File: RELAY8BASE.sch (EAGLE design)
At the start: 75 parts, among them IC1 MCP23017SO, J1 Analog, J2 POWER, J3 Digital_0_7, J4 M100.1, J5 ICSPPTH, J7 PWR SELECT, Q1 2N7002, Q2 2N7002, Q3 2N7002, Q4 2N7002, Q5 2N7002, Q6 2N7002, Q7 2N7002, Q8 2N7002

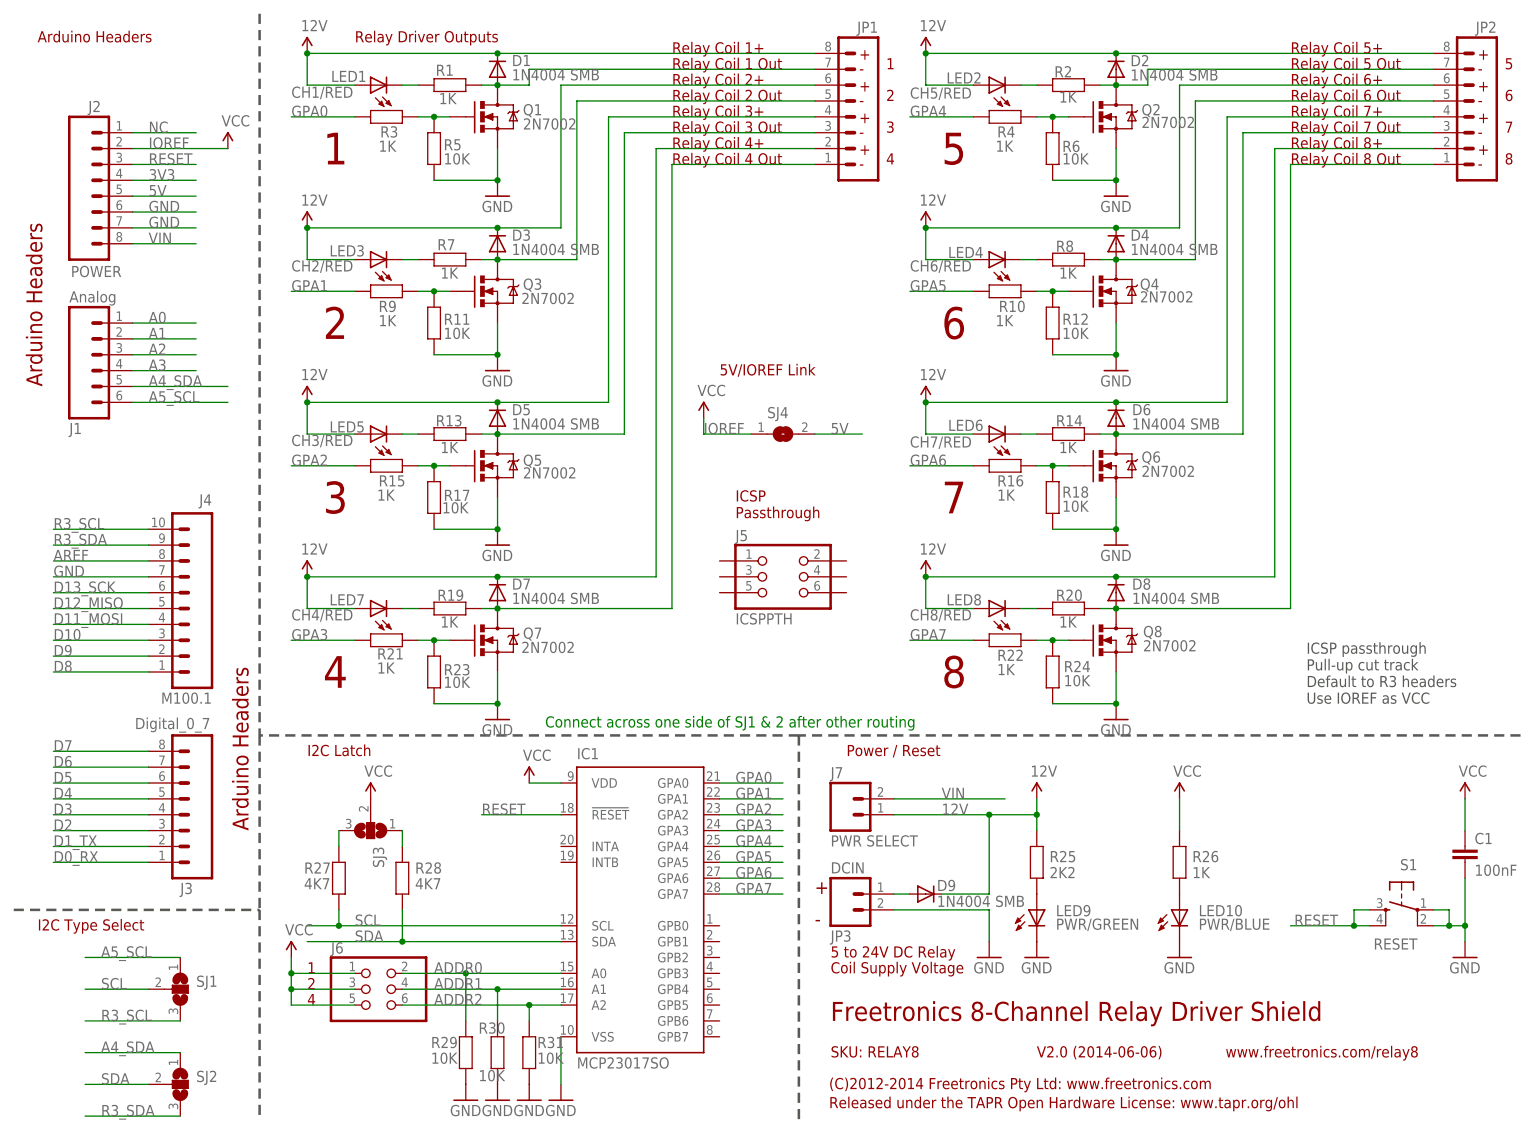
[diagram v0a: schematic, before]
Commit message: Layout for v1.0 release
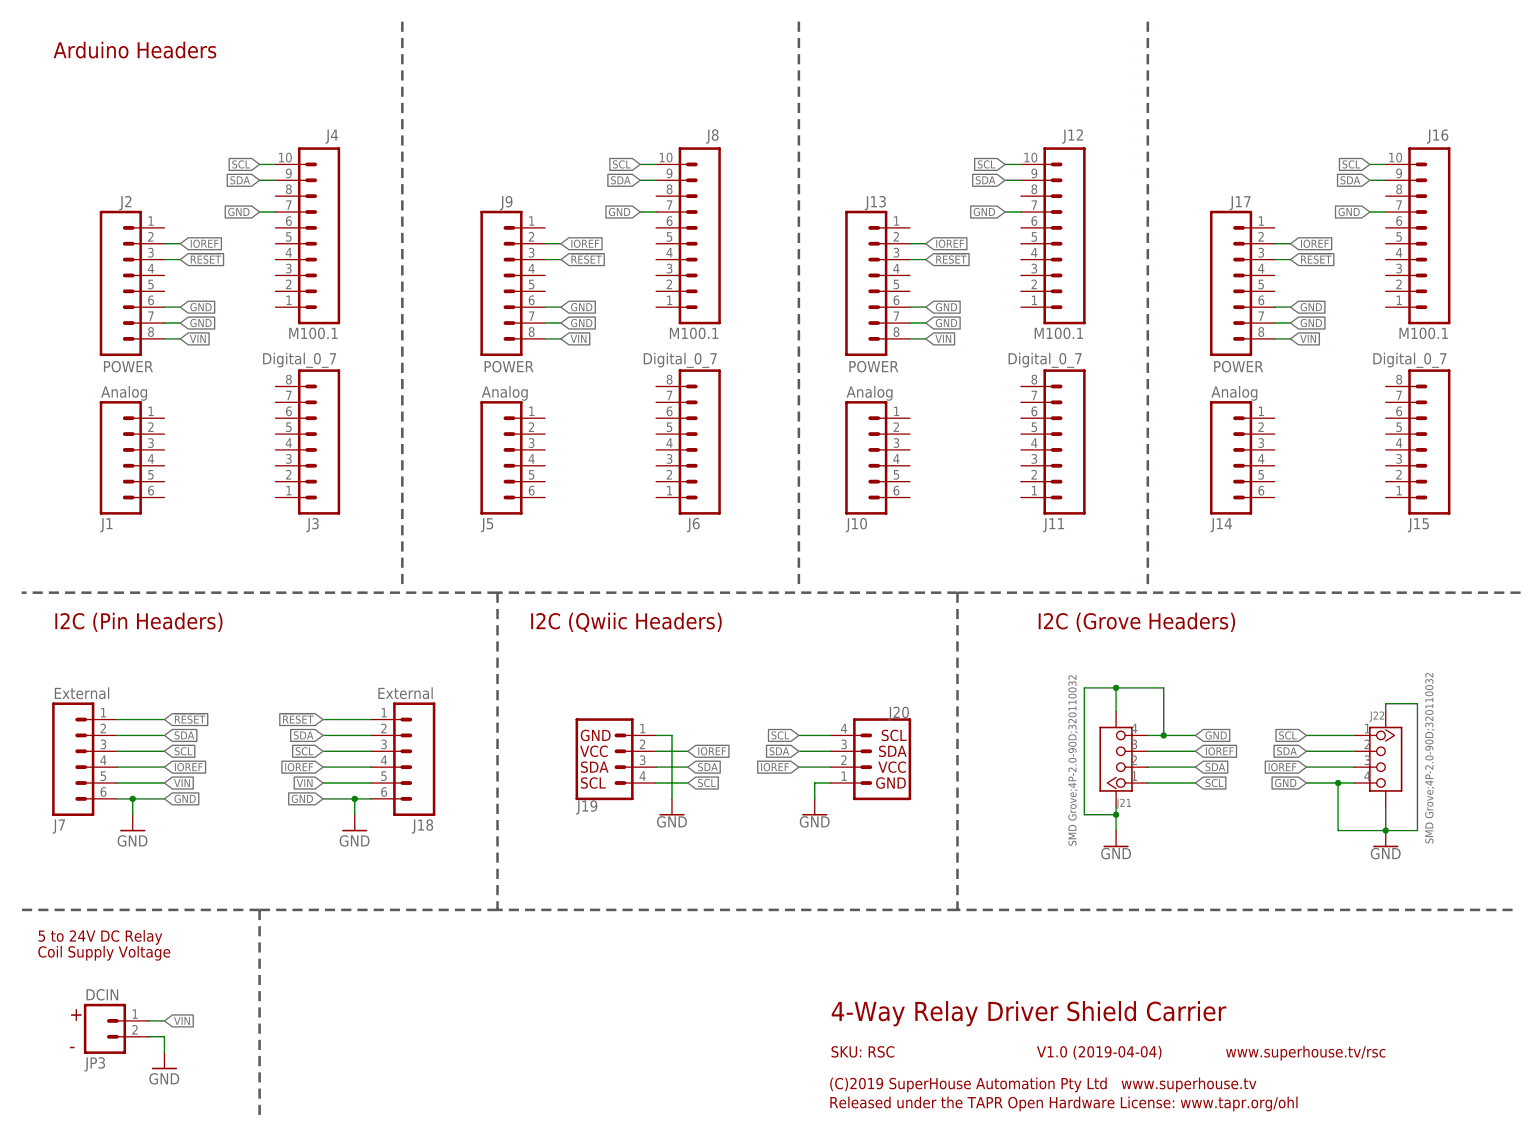
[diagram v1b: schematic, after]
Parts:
- removed C1: 100nF, freetronics-original:CAP0603
- removed D1, D2, D3, D4, D5, D6, D7, D8, D9: 1N4004 SMB, freetronics-master-v1.1:DIODESMB
- removed IC1: MCP23017SO, microchip:MCP23017SO
- removed JP1, JP2: (no value), freetronics-master-v1:M08
- removed LED1: CH1/RED, freetronics-master-v1:LED0603
- removed LED10: PWR/BLUE, freetronics-master-v1:LED0603
- removed LED2: CH5/RED, freetronics-master-v1:LED0603
- removed LED3: CH2/RED, freetronics-master-v1:LED0603
- removed LED4: CH6/RED, freetronics-master-v1:LED0603
- removed LED5: CH3/RED, freetronics-master-v1:LED0603
- removed LED6: CH7/RED, freetronics-master-v1:LED0603
- removed LED7: CH4/RED, freetronics-master-v1:LED0603
- removed LED8: CH8/RED, freetronics-master-v1:LED0603
- removed LED9: PWR/GREEN, freetronics-master-v1:LED0603
- removed Q1, Q2, Q3, Q4, Q5, Q6, Q7, Q8: 2N7002, freetronics-master-v1:MOSFET-NCHANNELSMD
- removed R1, R10, R13, R14, R15, R16, R19, R2, R20, R21, R22, R26, R3, R4, R7, R8, R9: 1K, freetronics-master-v1:RESISTOR0603
- removed R11, R12, R17, R18, R23, R24, R29, R30, R31, R5, R6: 10K, freetronics-master-v1:RESISTOR0603
- removed R25: 2K2, freetronics-master-v1:RESISTOR0603
- removed R27, R28: 4K7, freetronics-master-v1:RESISTOR0603
- removed S1: RESET, freetronics-original:TAC_SWITCHSMD
- removed SJ1, SJ2, SJ3: (no value), freetronics-master-v1.1:SJ2W
- removed SJ4: (no value), freetronics-jon:SJN
- added J10, J14: Analog, freetronics:M06SIP
- added J11, J15: Digital_0_7, freetronics:M08
- added J12, J16, J8: M100.1, freetronics-original:M100.1
- added J13, J17, J9: POWER, freetronics:M08
- added J18: External, freetronics:M06SIP
- added J19, J20: (no value), SparkFun-Connectors:QWIIC_CONNECTORJS-1MM
- added J21, J22: SMD Grove;4P-2.0-90D;320110032, Connector-new:GROVE-CONNECTOR-SMD'90D'
- J5: value ICSPPTH -> Analog; device freetronics-jon:ICSPPTH -> freetronics:M06SIP
- J6: value (none) -> Digital_0_7; device freetronics-master-v1.1:PINHD-2X3 -> freetronics:M08
- J7: value PWR SELECT -> External; device SparkFun:M02PTH -> freetronics:M06SIP
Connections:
- removed net 12V: D1.C, D2.C, D3.C, D4.C, D5.C, D6.C, D7.C, D8.C, D9.C, J7.1, JP1.2, JP1.4, JP1.6, JP1.8, JP2.2, JP2.4, JP2.6, JP2.8, LED1.A, LED2.A, LED3.A, LED4.A, LED5.A, LED6.A, LED7.A, LED8.A, R25.2
- removed net 3V3: J2.4
- removed net 5V: J2.5, SJ4.2
- removed net A0: J1.1
- removed net A1: J1.2
- removed net A2: J1.3
- removed net A3: J1.4
- removed net A4_SDA: J1.5, SJ2.1
- removed net A5_SCL: J1.6, SJ1.1
- removed net ADDR0: IC1.A0, J6.2, R29.2
- removed net ADDR1: IC1.A1, J6.4, R30.2
- removed net ADDR2: IC1.A2, J6.6, R31.2
- removed net AREF: J4.8
- removed net D0_RX: J3.1
- removed net D10: J4.3
- removed net D11_MOSI: J4.4
- removed net D12_MISO: J4.5
- removed net D13_SCK: J4.6
- removed net D1_TX: J3.2
- removed net D2: J3.3
- removed net D3: J3.4
- removed net D4: J3.5
- removed net D5: J3.6
- removed net D6: J3.7
- removed net D7: J3.8
- removed net D8: J4.1
- removed net D9: J4.2
- removed net GPA0: IC1.GPA0, R3.2
- removed net GPA1: IC1.GPA1, R9.2
- removed net GPA2: IC1.GPA2, R15.2
- removed net GPA3: IC1.GPA3, R21.2
- removed net GPA4: IC1.GPA4, R4.2
- removed net GPA5: IC1.GPA5, R10.2
- removed net GPA6: IC1.GPA6, R16.2
- removed net GPA7: IC1.GPA7, R22.2
- removed net N$1: Q1.G, R3.1, R5.2
- removed net N$10: Q5.G, R15.1, R17.2
- removed net N$11: D7.A, JP1.1, Q7.D, R19.2
- removed net N$12: Q7.G, R21.1, R23.2
- removed net N$13: D2.A, JP2.7, Q2.D, R2.2
- removed net N$14: Q2.G, R4.1, R6.2
- removed net N$15: D4.A, JP2.5, Q4.D, R8.2
- removed net N$16: Q4.G, R10.1, R12.2
- removed net N$17: D6.A, JP2.3, Q6.D, R14.2
- removed net N$18: Q6.G, R16.1, R18.2
- removed net N$19: D8.A, JP2.1, Q8.D, R20.2
- removed net N$20: Q8.G, R22.1, R24.2
- removed net N$21: LED3.C, R7.1
- removed net N$22: LED7.C, R19.1
- removed net N$23: LED5.C, R13.1
- removed net N$24: LED1.C, R1.1
- removed net N$25: LED2.C, R2.1
- removed net N$26: LED4.C, R8.1
- removed net N$27: LED6.C, R14.1
- removed net N$28: LED8.C, R20.1
- removed net N$3: D3.A, JP1.5, Q3.D, R7.2
- removed net N$4: LED9.A, R25.1
- removed net N$41: D9.A, JP3.1
- removed net N$42: R27.2, SJ3.3
- removed net N$43: R28.2, SJ3.1
- removed net N$5: D1.A, JP1.7, Q1.D, R1.2
- removed net N$52: LED10.A, R26.1
- removed net N$8: Q3.G, R11.2, R9.1
- removed net N$9: D5.A, JP1.3, Q5.D, R13.2
- removed net NC: J2.1
- removed net R3_SCL: J4.10, SJ1.3
- removed net R3_SDA: J4.9, SJ2.3
- removed net RESET: IC1.!RESET, J2.3, S1.3, S1.4
- new net !RESET: J13.3, J17.3, J18.1, J2.3, J7.1, J9.3
- net GND: now also J12.7, J13.6, J13.7, J16.7, J17.6, J17.7, J18.6, J19.1, J20.1, J21.4, J21.SS1, J21.SS2, J22.4, J22.SS1, J22.SS2, J7.6, J8.7, J9.6, J9.7; no longer C1.2, IC1.VSS, LED10.C, LED9.C, Q1.S, Q2.S, Q3.S, Q4.S, Q5.S, Q6.S, Q7.S, Q8.S, R11.1, R12.1, R17.1, R18.1, R23.1, R24.1, R29.1, R30.1, R31.1, R5.1, R6.1, S1.1, S1.2
- net IOREF: now also J13.2, J17.2, J18.4, J19.2, J20.2, J21.3, J22.3, J7.4, J9.2; no longer C1.1, IC1.VDD, J6.1, J6.3, J6.5, R26.2, SJ3.2, SJ4.1
- net SCL: now also J12.10, J16.10, J18.3, J19.4, J20.4, J21.1, J22.1, J4.10, J7.3, J8.10; no longer IC1.SCL, R27.1, SJ1.2
- net SDA: now also J12.9, J16.9, J18.2, J19.3, J20.3, J21.2, J22.2, J4.9, J7.2, J8.9; no longer IC1.SDA, R28.1, SJ2.2
- net VIN: now also J13.8, J17.8, J18.5, J7.5, J9.8, JP3.1; no longer J7.2
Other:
- note added: "(C)2019 SuperHouse Automation Pty Ltd www.superhouse.tv"
- note added: "4-Way Relay Driver Shield Carrier"
- note added: "I2C (Grove Headers)"
- note added: "I2C (Pin Headers)"
- note added: "I2C (Qwiic Headers)"
- note added: "SKU: RSC"
- note added: "V1.0 (2019-04-04)"
- note added: "www.superhouse.tv/rsc"
- note removed: "(C)2012-2014 Freetronics Pty Ltd: www.freetronics.com"
- note removed: "1"
- note removed: "2"
- note removed: "3"
- note removed: "4"
- note removed: "5"
- note removed: "5V/IOREF Link"
- note removed: "6"
- note removed: "7"
- note removed: "8"
- note removed: "Connect across one side of SJ1 & 2 after other routing"
- note removed: "Freetronics 8-Channel Relay Driver Shield"
- note removed: "I2C Latch"
- note removed: "I2C Type Select"
- note removed: "ICSP Passthrough"
- note removed: "ICSP passthrough Pull-up cut track Default to R3 headers Use IOREF as VCC"
- note removed: "Power / Reset"
- note removed: "Relay Coil 1 Out"
- note removed: "Relay Coil 1+"
- note removed: "Relay Coil 2 Out"
- note removed: "Relay Coil 2+"
- note removed: "Relay Coil 3 Out"
- note removed: "Relay Coil 3+"
- note removed: "Relay Coil 4 Out"
- note removed: "Relay Coil 4+"
- note removed: "Relay Coil 5 Out"
- note removed: "Relay Coil 5+"
- note removed: "Relay Coil 6 Out"
- note removed: "Relay Coil 6+"
- note removed: "Relay Coil 7 Out"
- note removed: "Relay Coil 7+"
- note removed: "Relay Coil 8 Out"
- note removed: "Relay Coil 8+"
- note removed: "Relay Driver Outputs"
- note removed: "SKU: RELAY8"
- note removed: "V2.0 (2014-06-06)"
- note removed: "www.freetronics.com/relay8"
- moved on the sheet: J1, J2, J3, J4, J5, JP3
